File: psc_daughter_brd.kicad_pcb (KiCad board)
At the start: 10 copper layers, 50 x 154.5 mm, 298 parts, among them J1 61082-061400LF, J2 61082-061400LF, U1 AD8221, U10 BUF634AxD, U11 BUF634AxD, U12 ADR1001AEZ, U13 ADS8568SPM, U14 AD8221, U15 OPA277, U16 AD8221, U17 OPA277, U18 AD8221, U19 OPA277, U2 OPA277, U20 LT3042xMSE, U26 LTC6655BHLS8-5, U27 AD8429BRZ, U28 AD8675ARZ, U29 LT6202CS5, U3 AD8676xR, U30 LTC6363xMS8, U31 LTC2376CDE-20-PBF, U32 LTC6655BHLS8-5, U33 AD8429BRZ, U34 AD8675ARZ, U35 LT6202CS5, U36 LTC6363xMS8, U37 LTC2376CDE-20-PBF, U38 TXUN0104RUTR, U39 ADUM5240ARZ, U4 AD8676xR, U40 ADUM5240ARZ, U41 TXUN0104RUTR, U42 ADUM5242ARZ, U43 ADUM5242ARZ, U5 AD5791BRUZ, U6 AD797, U7 OPA277, U8 OPA277, U9 OPA277

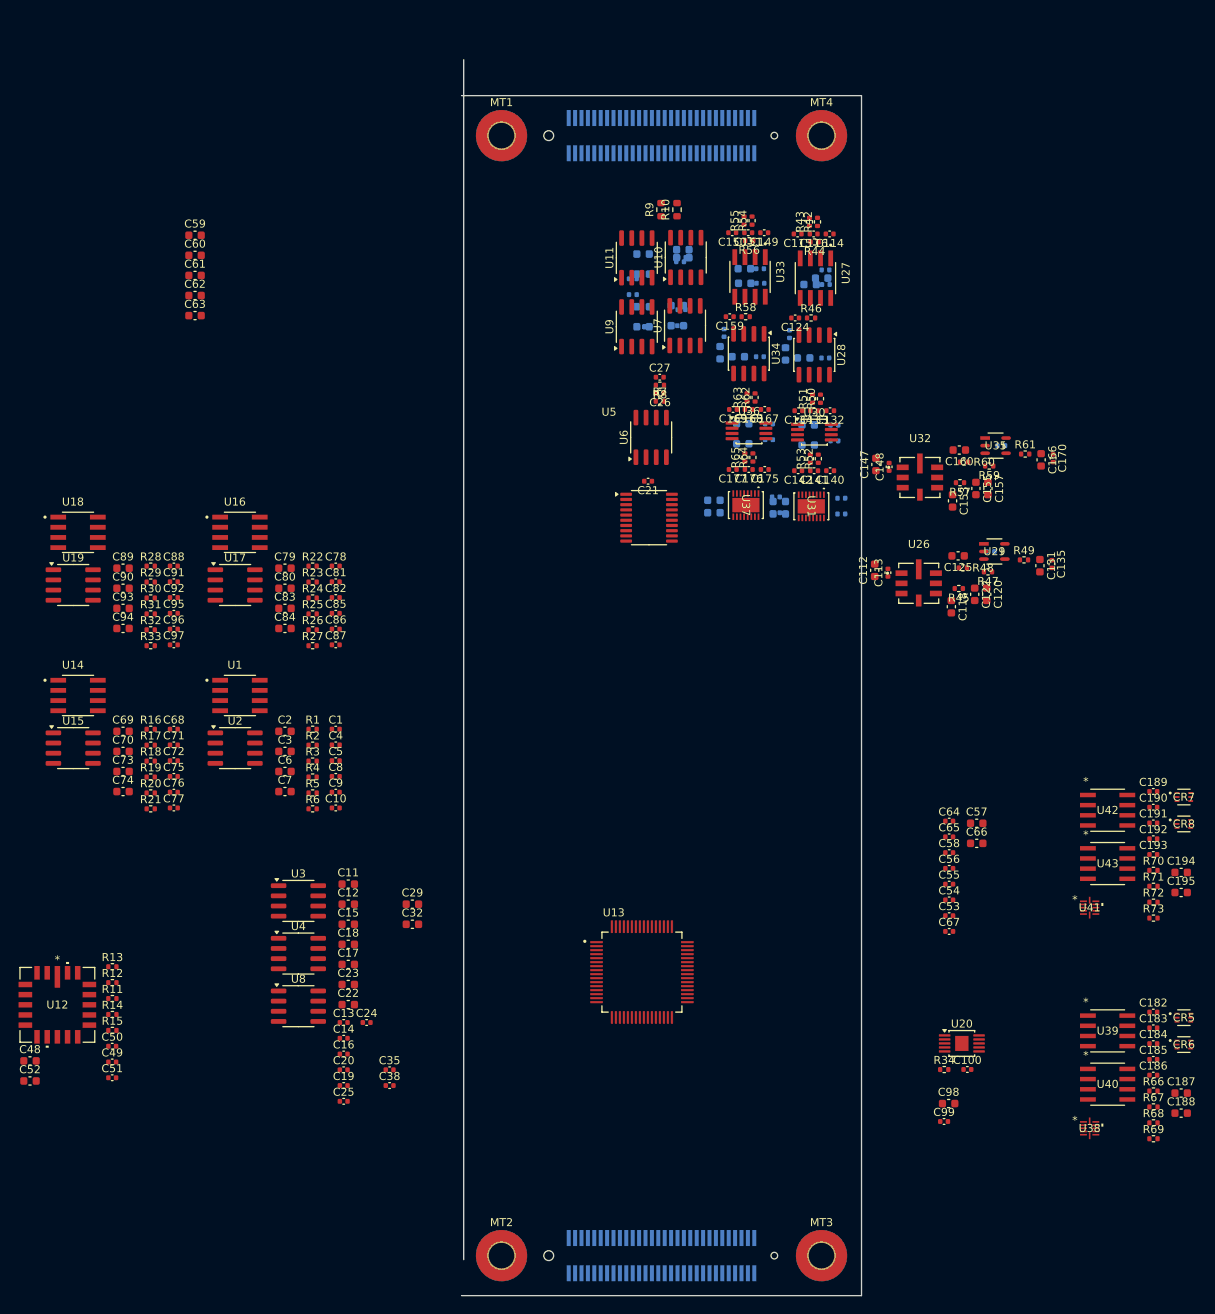
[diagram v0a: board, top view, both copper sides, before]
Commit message: finish rough placement
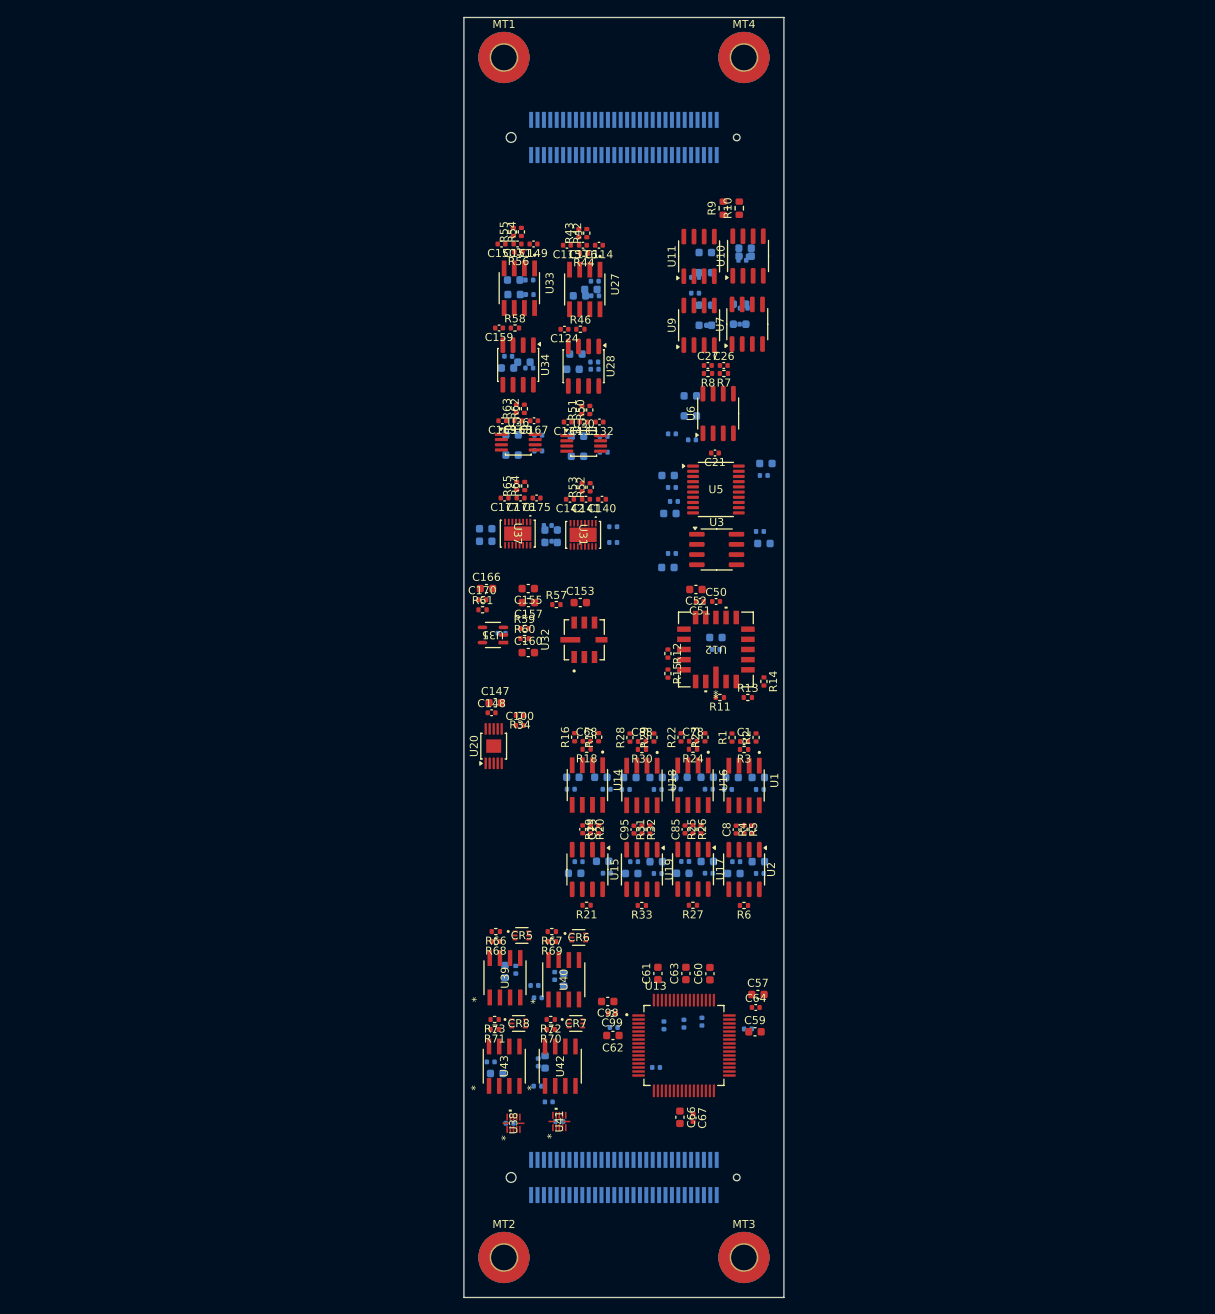
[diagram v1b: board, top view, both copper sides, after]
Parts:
- removed C112, C118, C120, C122, C125, C131, C29, C32: 10uF, Capacitor_SMD:C_0603_1608Metric
- removed C113, C129, C135, C35, C38: 0.1uF, Capacitor_SMD:C_0402_1005Metric
- removed R45: 0, Resistor_SMD:R_0402_1005Metric
- removed R47, R48: 10K, Resistor_SMD:R_0402_1005Metric
- removed R49: 10, Resistor_SMD:R_0402_1005Metric
- removed U26: LTC6655BHLS8-5, myparts:LTC6655
- removed U29: LT6202CS5, myparts:LT6202CS5
- removed U4: AD8676xR, Package_SO:SOIC-8_3.9x4.9mm_P1.27mm
- removed U8: OPA277, Package_SO:SOIC-8_3.9x4.9mm_P1.27mm
- C10, C11, C12, C13, C14, C15, C16, C17, C18, C182, C183, C184, C185, C186, C187, C188, C189, C19, C190, C191, C192, C193, C194, C195, C2, C20, C22, C23, C24, C25, C3, C4, C48, C49, C5, C53, C54, C55, C56, C58, C6, C65, C69, C7, C70, C71, C72, C73, C74, C76, C77, C79, C80, C81, C82, C83, C84, C86, C87, C89, C9, C90, C91, C92, C93, C94, C96, C97: moved to B.Cu
- moved C59 121.7 mm to (176.4, 158.8)
- moved C60 110.5 mm to (170.8, 151.5), turned to 90 degrees
- moved C62 106.2 mm to (158.6, 159.2), turned to 180 degrees
- moved C61 104.7 mm to (164.2, 151.5), turned to 90 degrees
- moved C52 103.5 mm to (169.0, 103.5), turned to 180 degrees
- moved C63 102.6 mm to (167.8, 151.5), turned to 90 degrees
- moved C48 100.8 mm to (171.5, 109.5)
- moved C51 94.6 mm to (169.5, 105.0), turned to 180 degrees
- moved C50 93.7 mm to (171.5, 105.0)
- moved U12 93.5 mm to (171.5, 111.0), turned to 180 degrees
- moved C25 93.4 mm to (168.5, 84.8), turned to 180 degrees
- moved C19 92.6 mm to (177.5, 89.2)
- moved R14 91.5 mm to (177.5, 115.0), turned to -90 degrees
- moved C49 91.4 mm to (171.5, 111.0)
- moved C195 88.5 mm to (144.1, 164.0)
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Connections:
- net /DCCT ADCs/DCCT Channel 1/vref_in renamed Net-(U20-OUT)
- C155 pad 1: Net-(U37-REF) -> /DCCT ADCs/DCCT Channel 1/adc_vref
- C157 pad 1: Net-(U37-REF) -> /DCCT ADCs/DCCT Channel 1/adc_vref
- C166 pad 1: Net-(U36-VOCM) -> /DCCT ADCs/DCCT Channel 1/drv_vref
- C170 pad 1: Net-(U36-VOCM) -> /DCCT ADCs/DCCT Channel 1/drv_vref
- C182 pad 1: +1V8 -> +1.8V
- J1 pad 10: /PS connector/digin_acon -> /Isolated Digital IO/din0_iso
- J1 pad 12: /PS connector/digin_flt1 -> /Isolated Digital IO/din1_iso
- J1 pad 14: /PS connector/digin_flt2 -> /Isolated Digital IO/din2_iso
- J1 pad 16: /PS connector/digin_spare -> /Isolated Digital IO/din3_iso
- J1 pad 2: /PS connector/digout_on1 -> /Isolated Digital IO/dout0_iso
- J1 pad 4: /PS connector/digout_on2 -> /Isolated Digital IO/dout1_iso
- J1 pad 6: /PS connector/digout_reset -> /Isolated Digital IO/dout2_iso
- J1 pad 8: /PS connector/digout_spare -> /Isolated Digital IO/dout3_iso
- R57 pad 1: Net-(U37-REF) -> /DCCT ADCs/DCCT Channel 1/adc_vref
- R59 pad 2: Net-(U37-REF) -> /DCCT ADCs/DCCT Channel 1/adc_vref
- R61 pad 1: Net-(U36-VOCM) -> /DCCT ADCs/DCCT Channel 1/drv_vref
- U3 pad 5: (no net) -> GND
- U3 pad 6: (no net) -> Net-(U3B--)
- U3 pad 7: (no net) -> Net-(U5-V_{REFNF})
- U30 pad 2: Net-(U30-VOCM) -> /DCCT ADCs/DCCT Channel 1/drv_vref
- U31 pad 7: Net-(U31-REF) -> /DCCT ADCs/DCCT Channel 1/adc_vref
- U31 pad 8: Net-(U31-REF) -> /DCCT ADCs/DCCT Channel 1/adc_vref
- U36 pad 2: Net-(U36-VOCM) -> /DCCT ADCs/DCCT Channel 1/drv_vref
- U37 pad 7: Net-(U37-REF) -> /DCCT ADCs/DCCT Channel 1/adc_vref
- U37 pad 8: Net-(U37-REF) -> /DCCT ADCs/DCCT Channel 1/adc_vref
- U38 pad 1: +1V8 -> +1.8V
- U5 pad 17: Net-(U4A--) -> Net-(U3B--)
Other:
- board size 50 x 154.5 mm -> 40 x 160 mm
